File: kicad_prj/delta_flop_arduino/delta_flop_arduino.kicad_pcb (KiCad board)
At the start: 2 copper layers, 116.7 x 59.9 mm, 21 parts, among them J1 SCREEN OUTPUT, J2 SD_Card, J3 Power Input (5V), J4 USB_C_Receptacle_PowerOnly_6P, SW1 RotaryEncoder_Switch, U1 Arduino_Nano

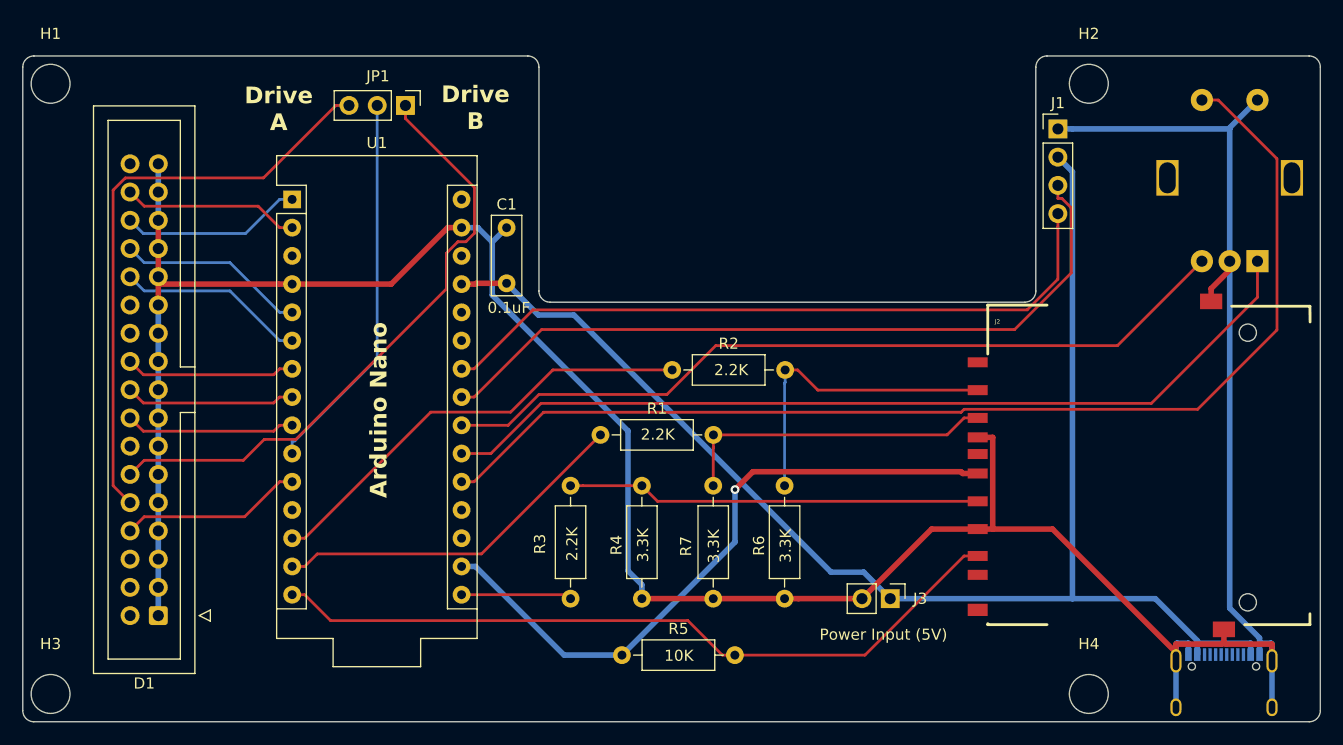
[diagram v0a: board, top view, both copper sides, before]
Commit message: Version 1.1 Update
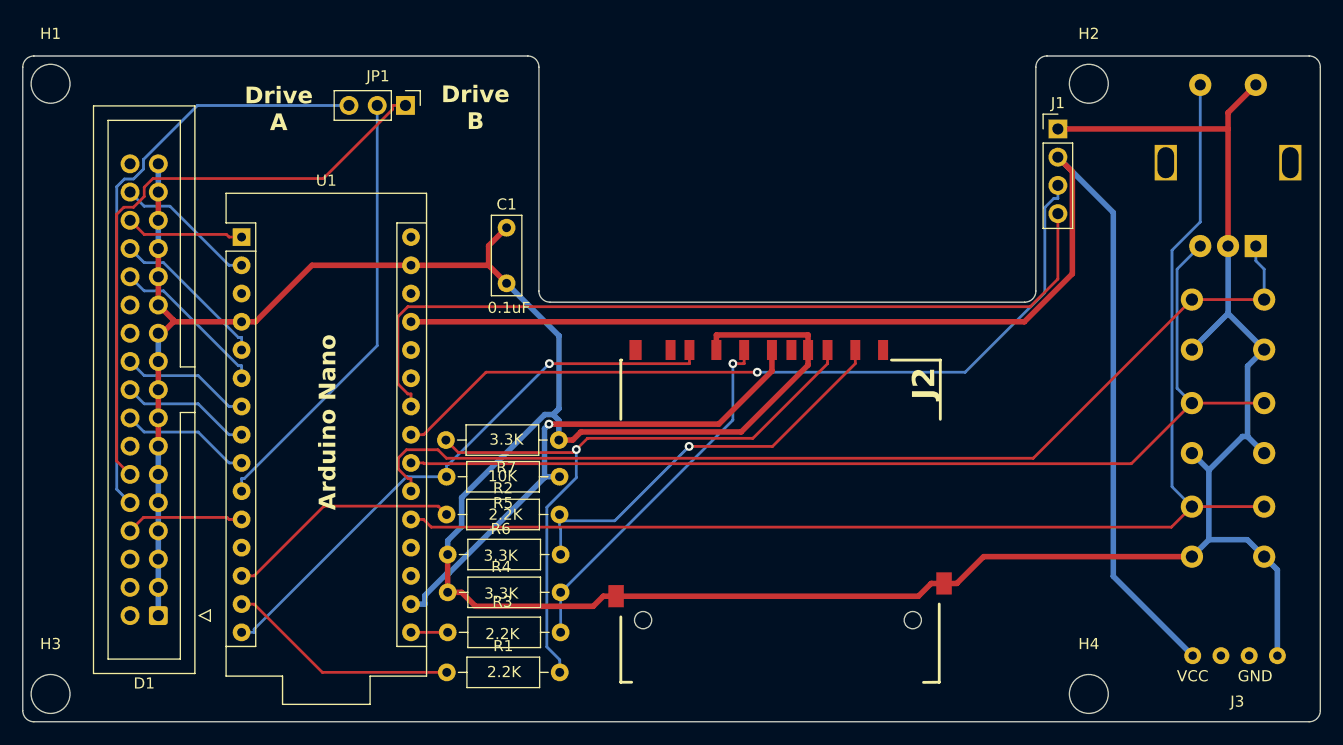
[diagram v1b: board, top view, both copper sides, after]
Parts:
- removed J4: USB_C_Receptacle_PowerOnly_6P, delta_flop_pre:USB_C_Receptacle_XKB_U262-16XN-4BVC11
- added SW2: Right, Button_Switch_THT:SW_PUSH_6mm, B.Cu at (214.9, 123.5)
- added SW3: Left, Button_Switch_THT:SW_PUSH_6mm, B.Cu at (214.9, 132.8)
- added SW4: Enter, Button_Switch_THT:SW_PUSH_6mm, B.Cu at (214.9, 142.1)
- J3: value Power Input (5V) -> Power connector; footprint Connector_PinHeader_2.54mm:PinHeader_1x02_P2.54mm_Vertical -> delta_flop_pre:USB-C Power board
- moved J3 31.5 mm to (212.4, 155.4), turned to 0 degrees
- moved R1 25.4 mm to (141.4, 157.0)
- moved R7 24.4 mm to (141.3, 136.1), turned to 0 degrees
- moved R2 24.1 mm to (141.4, 142.8)
- moved R6 21.1 mm to (151.7, 146.4), turned to 180 degrees
- moved J2 21.0 mm to (171.4, 129.0), turned to -90 degrees
- moved G*** 20.3 mm to (212.3, 150.8)
- moved R5 17.0 mm to (151.6, 139.4), turned to 180 degrees
- moved R4 12.1 mm to (151.7, 149.8), turned to 180 degrees
- moved R3 11.5 mm to (141.5, 153.4), turned to 0 degrees
- moved U1 5.67 mm to (123.0, 117.8)
- moved SW1 1.37 mm to (214.2, 118.7)
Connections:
- C1 pad 1: /5V -> GND
- J3 pad 2: GND -> unconnected-(J3-Pin_2-Pad2)
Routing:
- net GND: track 277.1 -> 309.4 mm
- net Net-(J2-CMD): track 29.0 -> 61.0 mm, vias 0 -> 1
- net Net-(U1-A3/D17): track 72.7 -> 94.6 mm
- net SS: track 40.5 -> 21.4 mm
- net MISO: track 67.6 -> 52.4 mm, vias 0 -> 1
- net Net-(U1-A1/D15): track 103.4 -> 117.5 mm
- net Net-(U1-A2/D16): track 80.7 -> 93.2 mm
- net Net-(J1-Pin_4): track 62.9 -> 75.4 mm
- net /3.3V: track 59.4 -> 47.4 mm
- net MOSI: track 32.6 -> 21.0 mm
- net Net-(J2-CD/DAT3): track 28.5 -> 37.3 mm, vias 0 -> 1
- net SCK: track 9.95 -> 3.30 mm
- net Net-(D1-INDEX): track 16.4 -> 10.6 mm
- net Net-(D1-READ_DATA): track 16.3 -> 10.7 mm
- net Net-(JP1-C): track 34.6 -> 39.9 mm
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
